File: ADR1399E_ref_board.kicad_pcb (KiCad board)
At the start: 4 copper layers, 119 x 60 mm, 103 parts, among them IC1 ADP7142ARDZ-R7, J1 Conn_01x02_Pin, J2 USB_C_Receptacle_PowerOnly_6P, J3 Conn_Coaxial, J4 S4B-XH-A, P1 JST_B2P_VH, Q1 MMBT3906, Q2 2N7002, U2 TPS61085DGK, U3 OPA182IDR, U4 OPA994IDR, U6 ADR1399KEZ, U7 LMT01LPG

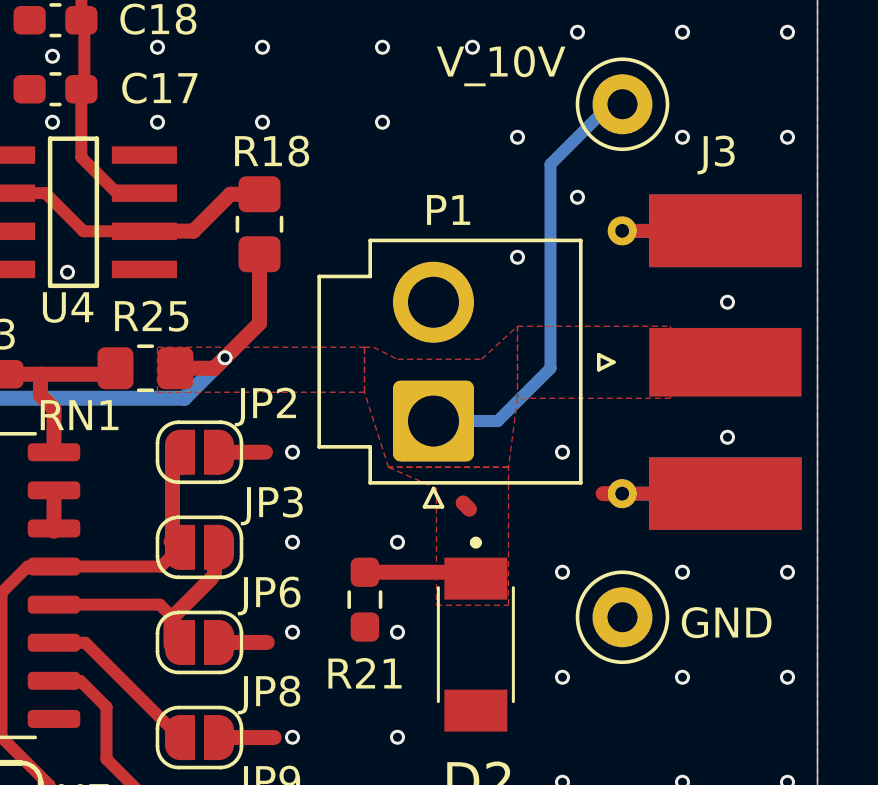
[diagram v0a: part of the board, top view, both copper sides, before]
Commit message: Update ADR1399E_ref_board.kicad_pcb
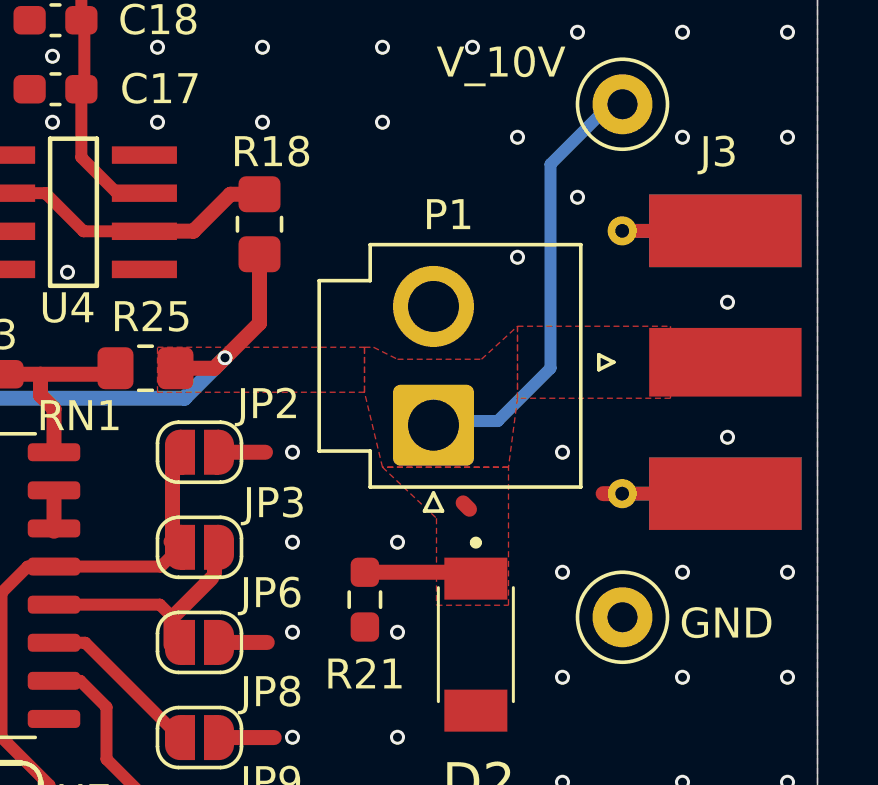
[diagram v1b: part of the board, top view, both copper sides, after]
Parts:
- moved P1 0.14 mm to (137.2, 106.1)
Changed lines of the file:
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@@
 	(footprint "Connector_JST:JST_VH_B2P-VH_1x02_P3.96mm_Vertical"
 		(layer "F.Cu")
-		(at 137.2 105.96 90)
+		(at 137.2 106.1 90)
 		(descr "JST VH series connector, B2P-VH (http://www.jst-mfg.com/product/pdf/eng/eVH.pdf), generated with kicad-footprint-generator")
 		(tags "connector JST VH vertical")
@@
 			(pts
 				(xy 134.9 103.5) (xy 135.2 103.5) (xy 136 103.9) (xy 138.8 103.9) (xy 140 102.8) (xy 140 105.2)
-				(xy 139.7 107.5) (xy 135.7 107.5) (xy 134.9 105)
+				(xy 139.7 107.5) (xy 135.5 107.5) (xy 134.9 105)
 			)
 		)
@@
 		(polygon
 			(pts
-				(xy 137.3 108.2) (xy 137.3 112.1) (xy 139.7 112.1) (xy 139.7 107.5) (xy 135.7 107.5)
+				(xy 137.3 109.2) (xy 137.3 112.1) (xy 139.7 112.1) (xy 139.7 107.5) (xy 135.5 107.5)
 			)
 		)
